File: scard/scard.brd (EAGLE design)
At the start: 90 x 74.5 mm, 72 parts, among them Q1 FDN360P, X1 COAX, X2 1365-20

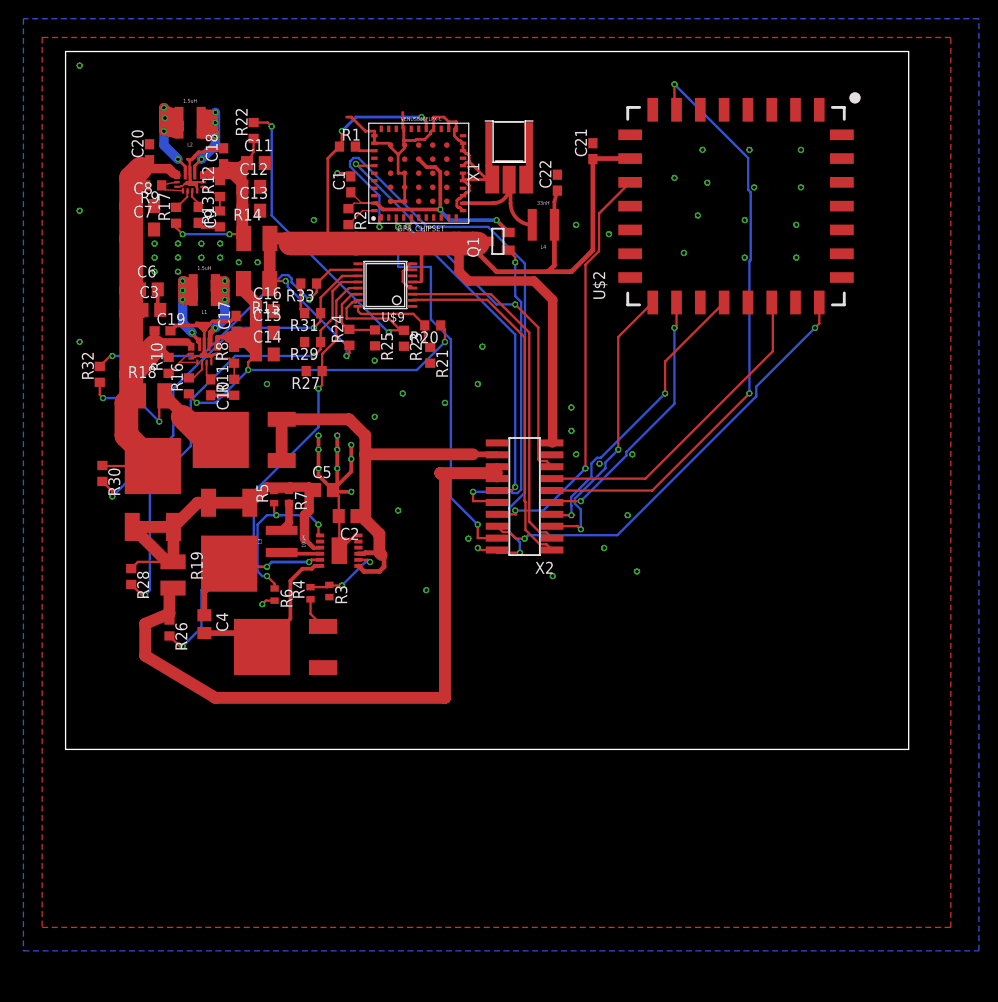
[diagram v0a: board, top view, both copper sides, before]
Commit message: changes from design review
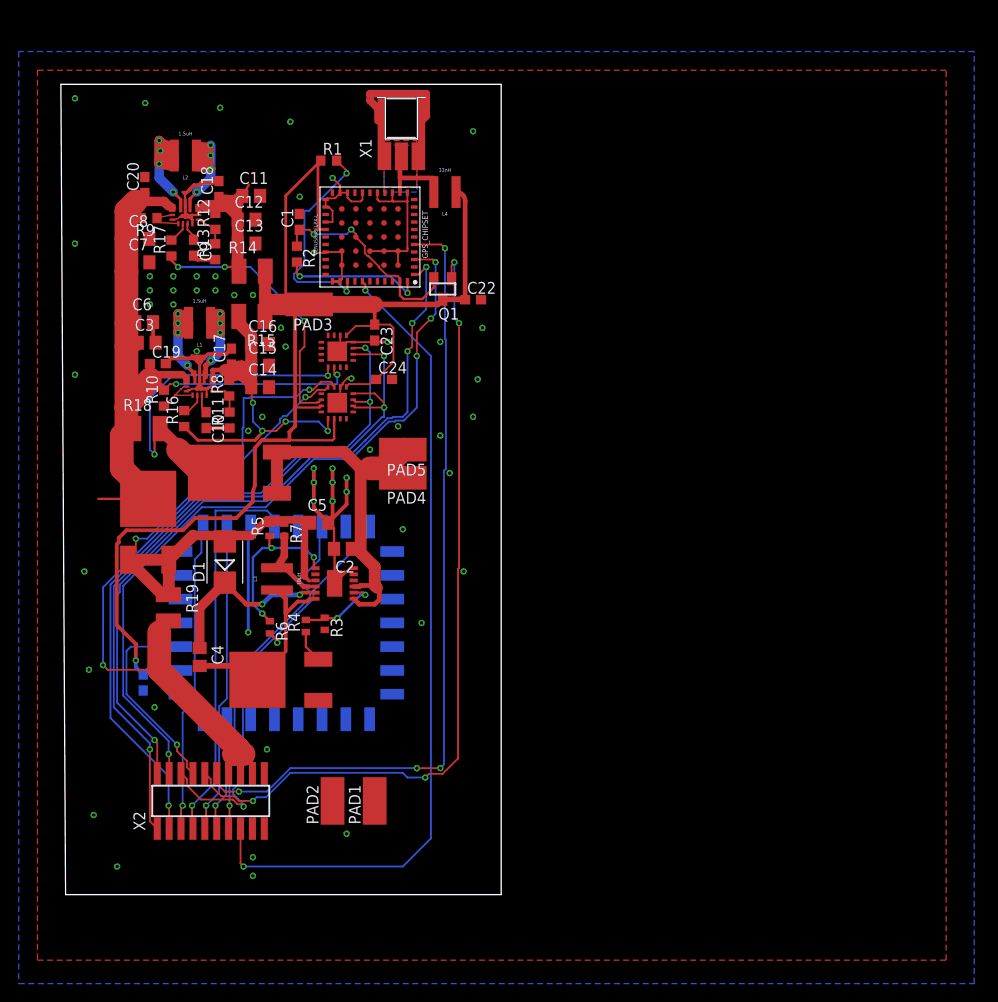
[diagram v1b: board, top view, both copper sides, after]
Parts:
- removed R20, R21, R22, R23, R24, R25, R27, R29, R31, R33: 1k, resistor:R0603
- removed R26, R28: 4k, resistor:R0603
- removed R30, R32: 5k, resistor:R0603
- removed U$3: B085BM30, calsat:TO-252
- removed U$9: ADC128D818, adc:ADC12_SD
- added A1, A3: INA3221-Q1, calsat:VQFN16
- added C23, C24: 0.1uF, resistor:C0603
- added D1: ES2D, diode:SMB
- added PAD1, PAD2, PAD3, PAD4, PAD5: (no value), wirepad:SMD2,54-5,08
- moved C21 74.3 mm to (8.29, 22.6), flipped to the bottom, turned to 270 degrees
- moved U$2 65.6 mm to (23.6, 28.9), flipped to the bottom, turned to 270 degrees
- moved X2 46.7 mm to (15.5, 10.0), turned to 0 degrees
- moved C22 15.4 mm to (43.5, 63.5), turned to 0 degrees
- moved X1 11.8 mm to (35.9, 85.0)
- moved L4 11.1 mm to (40.5, 75.0)
- moved GPS_CHIPSET 8.57 mm to (32.5, 70.2), turned to 270 degrees
- moved Q1 7.78 mm to (40.3, 64.7), turned to 180 degrees
- moved C1 6.80 mm to (24.9, 71.8)
- moved R2 6.80 mm to (24.7, 68.4)
- moved L3 4.03 mm to (22.6, 33.7)
- moved L1 3.54 mm to (14.3, 61.0)
- moved C10 3.54 mm to (15.0, 50.6)
- moved C11 3.54 mm to (19.8, 74.6)
- moved C12 3.54 mm to (19.3, 72.0)
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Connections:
- removed net N$16: R20.2, R21.1, U$9.16
- removed net N$17: R22.2, R23.1, U$9.15
- removed net N$18: R24.2, R25.1, U$9.14
- removed net N$19: R26.2, R27.1, U$9.13
- removed net N$2: CHRG_IC.10, L3.1
- removed net N$20: R28.2, R29.1, U$9.12
- removed net N$21: R30.2, R31.1, U$9.11
- removed net N$23: R32.2, R33.1, U$9.10
- new net N$32: A3.15
- new net N$33: A3.14
- new net N$34: A3.2
- new net N$35: A3.1
- net +12V: now also PAD4.1, PAD5.1; no longer X2.18
- net +3V3: now also A1.11, A1.14, A1.4, A3.4, C23.1, C24.1, PAD3.1; no longer R24.1, U$9.5, X2.19
- net GND: now also A1.17, A1.3, A3.17, A3.3, A3.5, C23.2, C24.2, PAD1.1, PAD2.1, X2.19; no longer R21.2, R23.2, R25.2, R27.2, R29.2, R31.2, R33.2, U$9.4, U$9.7, U$9.8
- net I2C_SCL: now also A1.6, A3.6; no longer U$9.3
- net I2C_SDA: now also A1.5, A1.7, A3.7; no longer U$9.2
- net N$3: now also D1.C; no longer U$3.1
- net N$4: now also L3.1
- net N$6: now also CHRG_IC.10
- net REG0_3V3: now also A1.12; no longer R20.1
- net REG1_3V3: now also A1.15; no longer R22.1
- net SYS_UNREG: now also A3.11; no longer R30.1
- net SYS_UNREG_CUR: now also A3.12; no longer R32.1
- net VBATT: now also A1.1, X2.18; no longer R26.1
- net VBATT_CUR: now also A1.2, D1.A; no longer R28.1, U$3.2, U$3.3
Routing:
- net TARE_GPIO: track 64.6 -> 12.2 mm, vias 2 -> 1
- net GPS_EN: track 35.1 -> 86.0 mm, vias 2 -> 4
- net N$20: track 50.7 -> 0.00 mm, vias 2 -> 0
- net P1PPS: track 35.8 -> 85.6 mm, vias 2 -> 4
- net N$19: track 48.4 -> 0.00 mm, vias 2 -> 0
- net I2C_SDA: track 38.0 -> 81.6 mm, vias 0 -> 3
- net STS: track 44.6 -> 87.9 mm
- net N$21: track 42.4 -> 0.00 mm, vias 2 -> 0
- net N$17: track 40.3 -> 0.00 mm, vias 2 -> 0
- net UART0_TXD: track 42.0 -> 80.0 mm, vias 2 -> 4
- net I2C_SCL: track 37.5 -> 75.0 mm, vias 0 -> 3
- net N$23: track 34.8 -> 0.00 mm, vias 2 -> 0
- net VBATT_CUR: track 45.8 -> 75.9 mm, vias 0 -> 2
- net IMU_EN: track 44.3 -> 21.9 mm, vias 2 -> 1
- net REG1_3V3: track 31.4 -> 52.2 mm, vias 2 -> 3
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- added copper zone on layer 1, net NONE
- added copper zone on layer 16, net NONE
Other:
- board size 90 x 74.5 mm -> 47 x 86.5 mm
